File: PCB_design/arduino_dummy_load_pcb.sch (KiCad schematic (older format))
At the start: 17 parts, among them J1 Barrel_Jack, J2 Conn_02x08_Odd_Even, M1 REG, U3 MCP3208

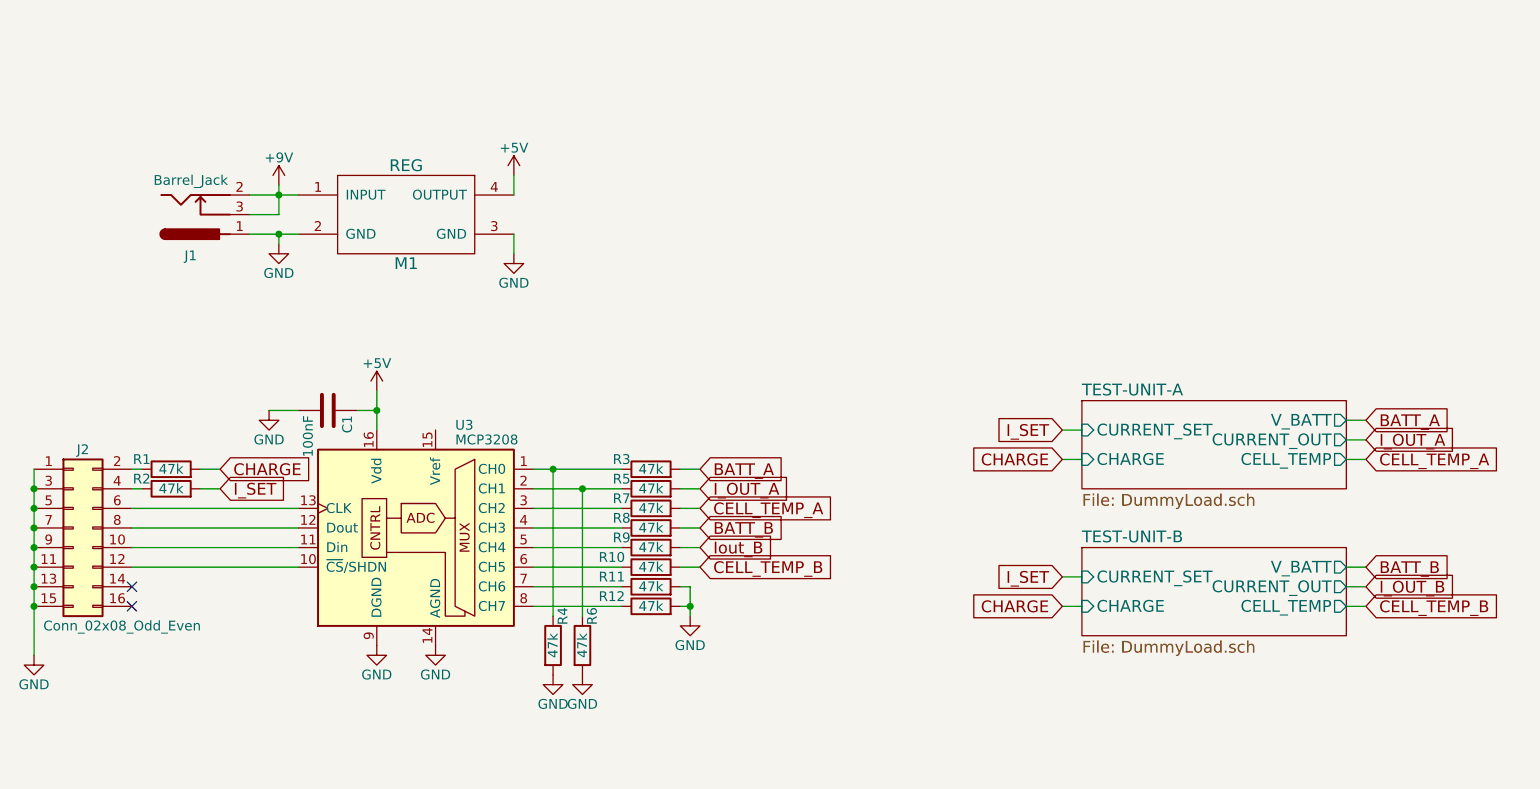
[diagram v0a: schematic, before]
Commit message: stuff.
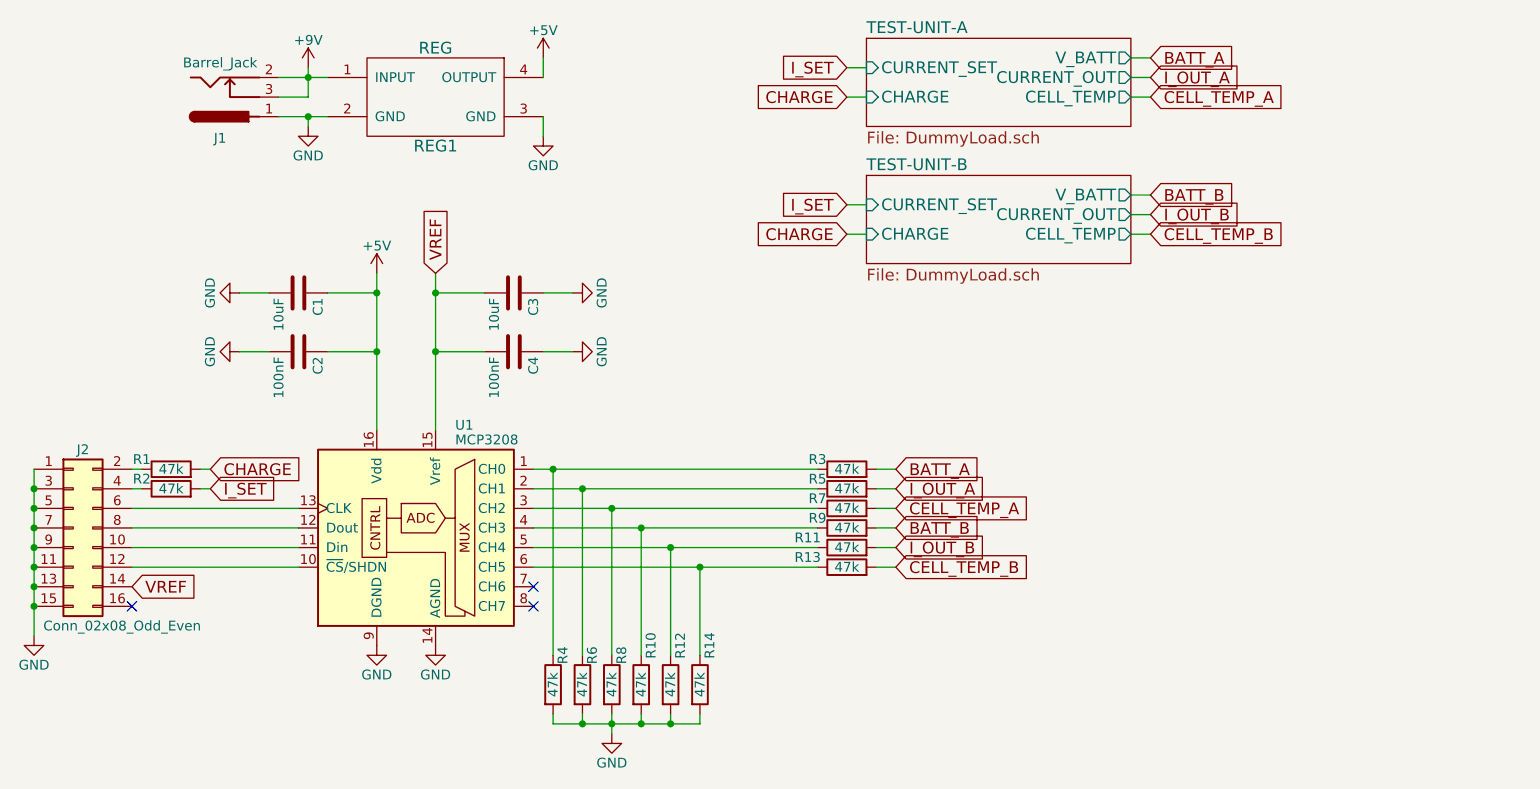
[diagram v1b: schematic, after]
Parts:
- added C2, C4: 100nF, Capacitors_SMD:C_0805_HandSoldering, symbol C
- added C3: 10uF, Capacitors_SMD:C_0805_HandSoldering, symbol C
- added R13, R14: 47k, Resistors_SMD:R_0805_HandSoldering, symbol R
- C1: value 100nF -> 10uF
- J2: footprint (none) -> Connectors:he10-16d
- U1: renamed from U3; footprint (none) -> Housings_SOIC:SOIC-16_3.9x9.9mm_Pitch1.27mm
- renumbered M1 to REG1
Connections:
- net Iout_B is gone; now on net BATT_B: R9.2
- net +5V: now also C2.1
- net BATT_B: no longer R8.2
- net CELL_TEMP_B: now also R13.2; no longer R10.2
- net GND: now also R10.2, R8.2, C2.2, C3.1, C4.1, R14.2; no longer R11.2
- net I_OUT_B: now also R11.2
- net VREF: now reaches U1.15 (Vref)
- net VREF: now also J2.14 (Pin_14), C3.2, C4.2
- net at R7.1, U1.3 (CH2): now also R8.1
- net at U1.4 (CH3): now also R10.1, R9.1; no longer R8.1
- net at U1.5 (CH4): now also R11.1, R12.1; no longer R9.1
- net at U1.6 (CH5): now also R13.1, R14.1; no longer R10.1
- net at U1.7 (CH6): no longer R11.1
- net at U1.8 (CH7): no longer R12.1
- no-connect marks 2 -> 3
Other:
- moved on the sheet: C1, J1, R10, R11, R12, R3, R4, R5, R6, R7, R8, R9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
